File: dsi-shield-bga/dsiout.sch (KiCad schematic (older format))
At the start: 12 parts

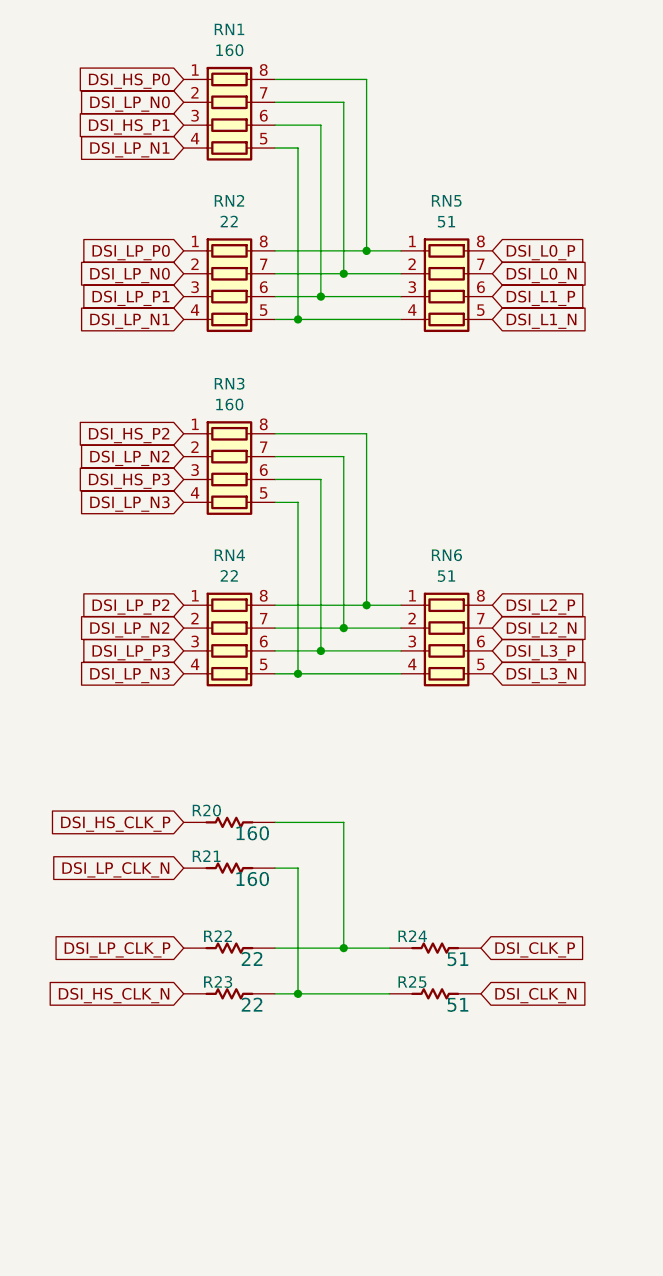
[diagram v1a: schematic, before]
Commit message: 20200719-1
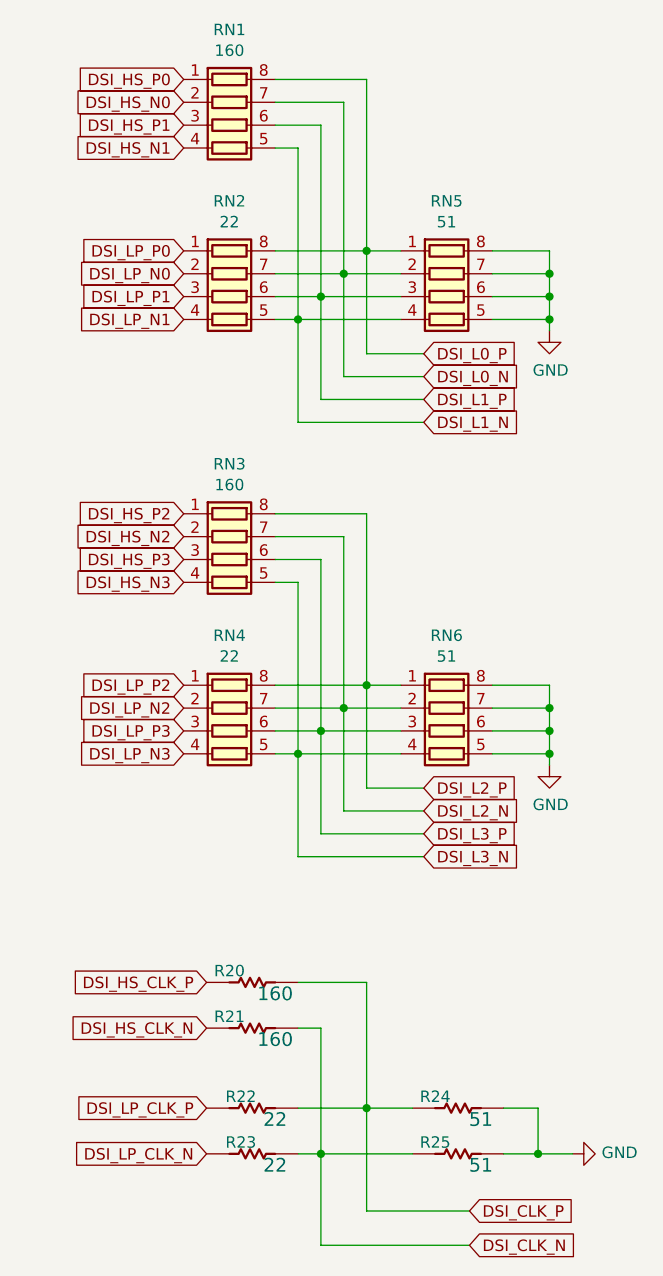
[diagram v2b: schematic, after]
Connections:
- net DSI_CLK_N: now also R21.2, R23.2, R25.1; no longer R25.2
- net DSI_CLK_P: now also R20.2, R22.2, R24.1; no longer R24.2
- net DSI_HS_CLK_N: now also R21.1; no longer R23.1
- net DSI_L0_N: now also RN1.7 (R2.2), RN2.7 (R2.2), RN5.2 (R2.1); no longer RN5.7 (R2.2)
- net DSI_L0_P: now also RN1.8 (R1.2), RN2.8 (R1.2), RN5.1 (R1.1); no longer RN5.8 (R1.2)
- net DSI_L1_N: now also RN1.5 (R4.2), RN2.5 (R4.2), RN5.4 (R4.1); no longer RN5.5 (R4.2)
- net DSI_L1_P: now also RN1.6 (R3.2), RN2.6 (R3.2), RN5.3 (R3.1); no longer RN5.6 (R3.2)
- net DSI_L2_N: now also RN3.7 (R2.2), RN4.7 (R2.2), RN6.2 (R2.1); no longer RN6.7 (R2.2)
- net DSI_L2_P: now also RN3.8 (R1.2), RN4.8 (R1.2), RN6.1 (R1.1); no longer RN6.8 (R1.2)
- net DSI_L3_N: now also RN3.5 (R4.2), RN4.5 (R4.2), RN6.4 (R4.1); no longer RN6.5 (R4.2)
- net DSI_L3_P: now also RN3.6 (R3.2), RN4.6 (R3.2), RN6.3 (R3.1); no longer RN6.6 (R3.2)
- net DSI_LP_CLK_N: now also R23.1; no longer R21.1
- net DSI_LP_N0: no longer RN1.2 (R2.1)
- net DSI_LP_N1: no longer RN1.4 (R4.1)
- net DSI_LP_N2: no longer RN3.2 (R2.1)
- net DSI_LP_N3: no longer RN3.4 (R4.1)
- new net DSI_HS_N0: RN1.2 (R2.1)
- new net DSI_HS_N1: RN1.4 (R4.1)
- new net DSI_HS_N2: RN3.2 (R2.1)
- new net DSI_HS_N3: RN3.4 (R4.1)
- new net GND: R24.2, R25.2, RN5.5 (R4.2), RN5.6 (R3.2), RN5.7 (R2.2), RN5.8 (R1.2), RN6.5 (R4.2), RN6.6 (R3.2), RN6.7 (R2.2), RN6.8 (R1.2)
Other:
- moved on the sheet: R20, R21, R22, R23, R24, R25, RN3, RN4, RN6

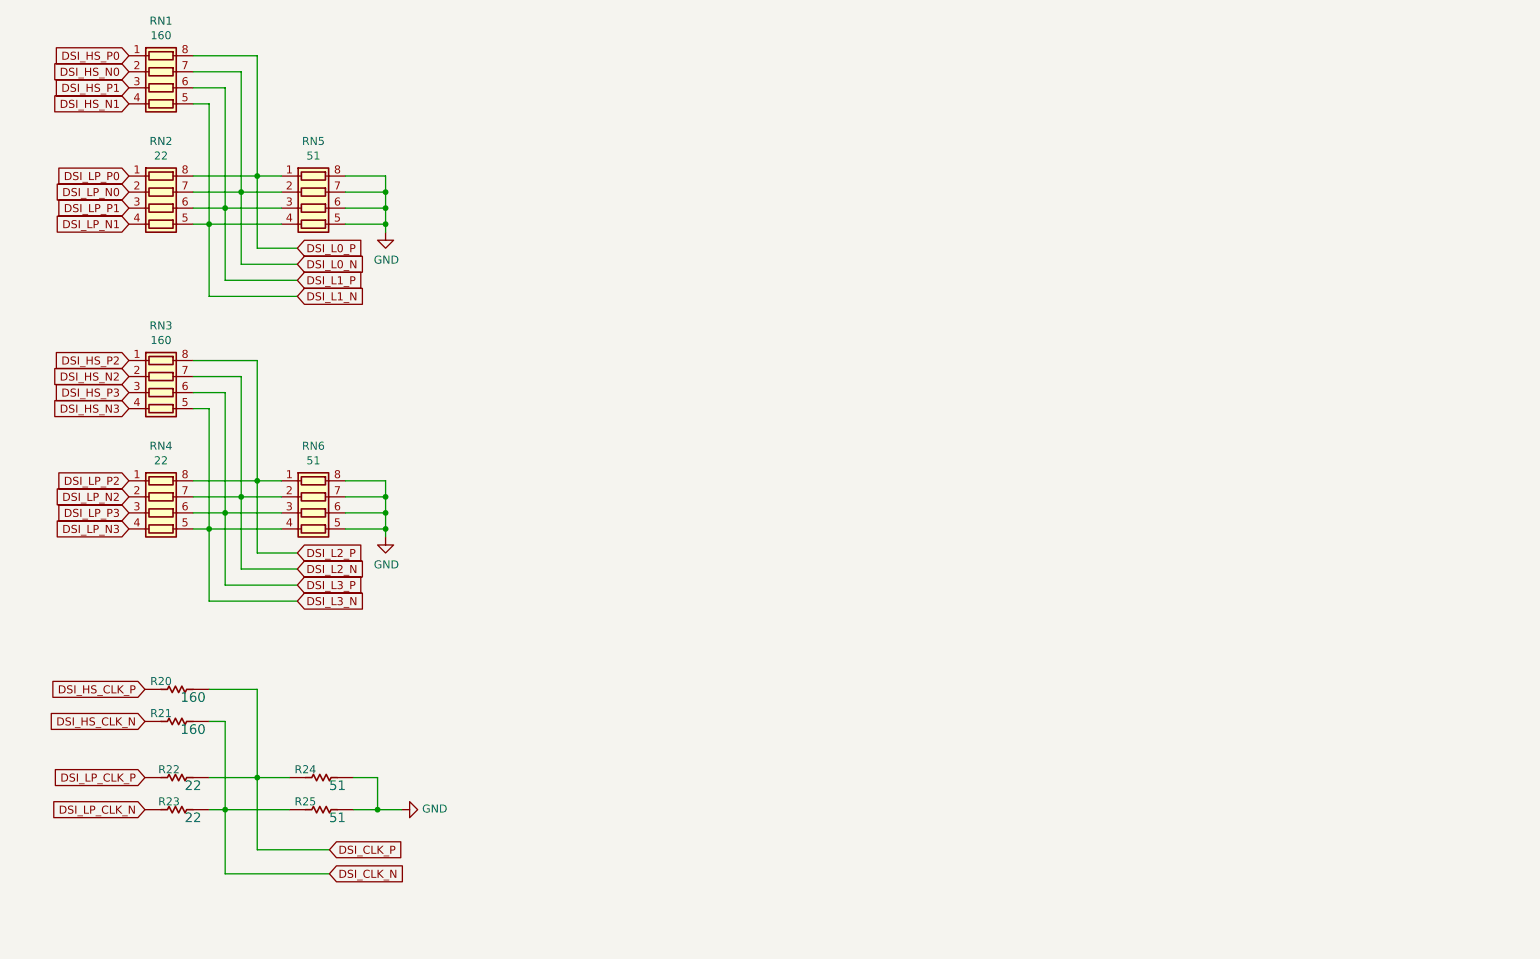
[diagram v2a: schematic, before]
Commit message: 20200808
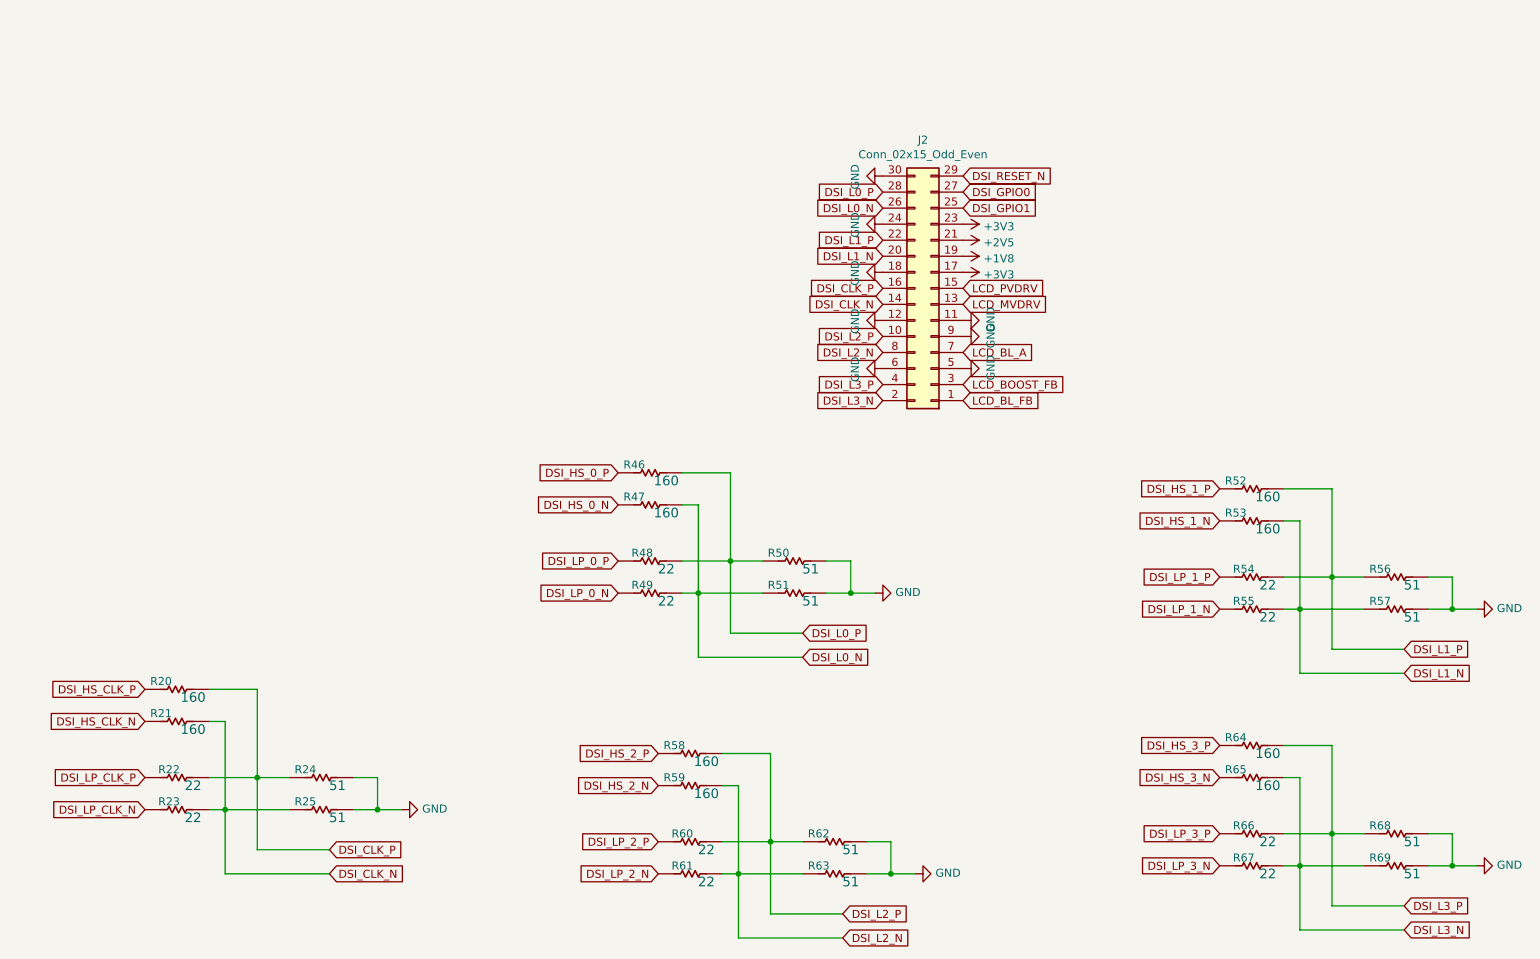
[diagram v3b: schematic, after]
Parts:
- removed RN1, RN3: 160, Resistor_SMD:R_Array_Convex_4x0402, symbol Device:R_Pack04
- removed RN2, RN4: 22, Resistor_SMD:R_Array_Convex_4x0402, symbol Device:R_Pack04
- removed RN5, RN6: 51, Resistor_SMD:R_Array_Convex_4x0402, symbol Device:R_Pack04
- added J2: Conn_02x15_Odd_Even, Connector_PinHeader_2.54mm:PinHeader_2x15_P2.54mm_Vertical, symbol Connector_Generic:Conn_02x15_Odd_Even
- added R46, R47, R52, R53, R58, R59, R64, R65: 160, Resistor_SMD:R_0402_1005Metric, symbol dsi_shield:Res1
- added R48, R49, R54, R55, R60, R61, R66, R67: 22, Resistor_SMD:R_0402_1005Metric, symbol dsi_shield:Res1
- added R50, R51, R56, R57, R62, R63, R68, R69: 51, Resistor_SMD:R_0402_1005Metric, symbol dsi_shield:Res1
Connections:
- net DSI_CLK_N: now also J2.14 (Pin_14)
- net DSI_CLK_P: now also J2.16 (Pin_16)
- net DSI_L0_N: now also J2.26 (Pin_26), R47.2, R49.2, R51.1
- net DSI_L0_P: now also J2.28 (Pin_28), R46.2, R48.2, R50.1
- net DSI_L1_N: now also J2.20 (Pin_20), R53.2, R55.2, R57.1
- net DSI_L1_P: now also J2.22 (Pin_22), R52.2, R54.2, R56.1
- net DSI_L2_N: now also J2.8 (Pin_8), R59.2, R61.2, R63.1
- net DSI_L2_P: now also J2.10 (Pin_10), R58.2, R60.2, R62.1
- net DSI_L3_N: now also J2.2 (Pin_2), R65.2, R67.2, R69.1
- net DSI_L3_P: now also J2.4 (Pin_4), R64.2, R66.2, R68.1
- net GND: now also J2.11 (Pin_11), J2.12 (Pin_12), J2.18 (Pin_18), J2.24 (Pin_24), J2.30 (Pin_30), J2.5 (Pin_5), J2.6 (Pin_6), J2.9 (Pin_9), R50.2, R51.2, R56.2, R57.2, R62.2, R63.2, R68.2, R69.2
- new net +1V8: J2.19 (Pin_19)
- new net +2V5: J2.21 (Pin_21)
- new net +3V3: J2.17 (Pin_17), J2.23 (Pin_23)
- new net DSI_GPIO0: J2.27 (Pin_27)
- new net DSI_GPIO1: J2.25 (Pin_25)
- new net DSI_HS_0_N: R47.1
- new net DSI_HS_0_P: R46.1
- new net DSI_HS_1_N: R53.1
- new net DSI_HS_1_P: R52.1
- new net DSI_HS_2_N: R59.1
- new net DSI_HS_2_P: R58.1
- new net DSI_HS_3_N: R65.1
- new net DSI_HS_3_P: R64.1
- new net DSI_LP_0_N: R49.1
- new net DSI_LP_0_P: R48.1
- new net DSI_LP_1_N: R55.1
- new net DSI_LP_1_P: R54.1
- new net DSI_LP_2_N: R61.1
- new net DSI_LP_2_P: R60.1
- new net DSI_LP_3_N: R67.1
- new net DSI_LP_3_P: R66.1
- new net DSI_RESET_N: J2.29 (Pin_29)
- new net LCD_BL_A: J2.7 (Pin_7)
- new net LCD_BL_FB: J2.1 (Pin_1)
- new net LCD_BOOST_FB: J2.3 (Pin_3)
- new net LCD_MVDRV: J2.13 (Pin_13)
- new net LCD_PVDRV: J2.15 (Pin_15)
